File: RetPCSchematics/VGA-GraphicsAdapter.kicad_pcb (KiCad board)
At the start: 2 copper layers, 200.7 x 104.1 mm, 27 parts, among them U501 TFP410, U8 SN74LVC245AN, X1 DGOF5S3

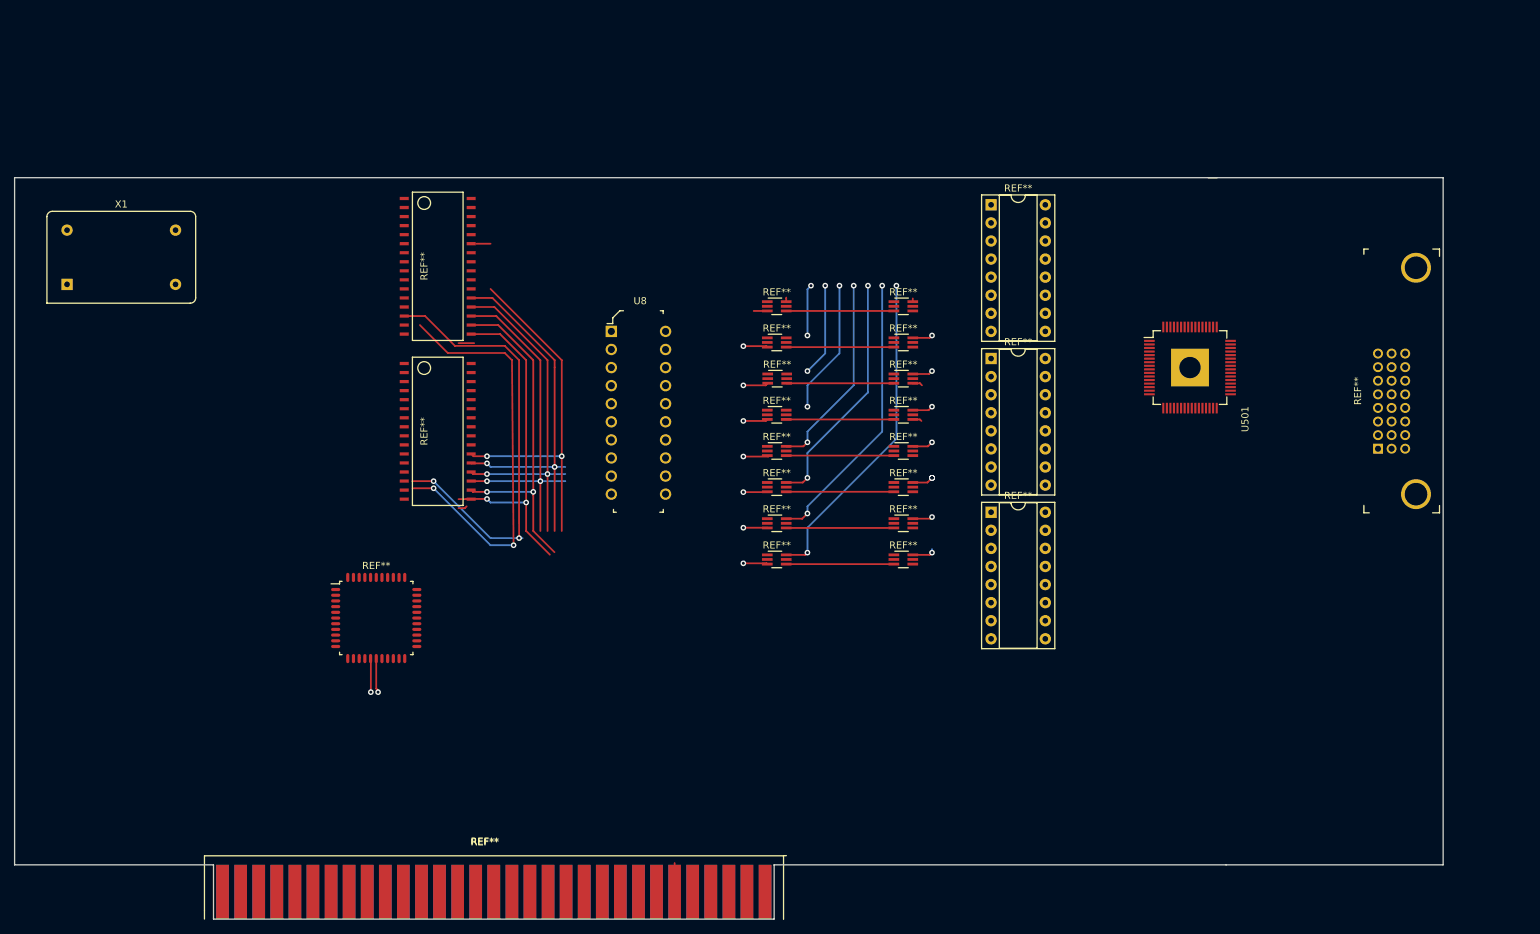
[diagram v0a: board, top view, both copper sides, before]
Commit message: sync
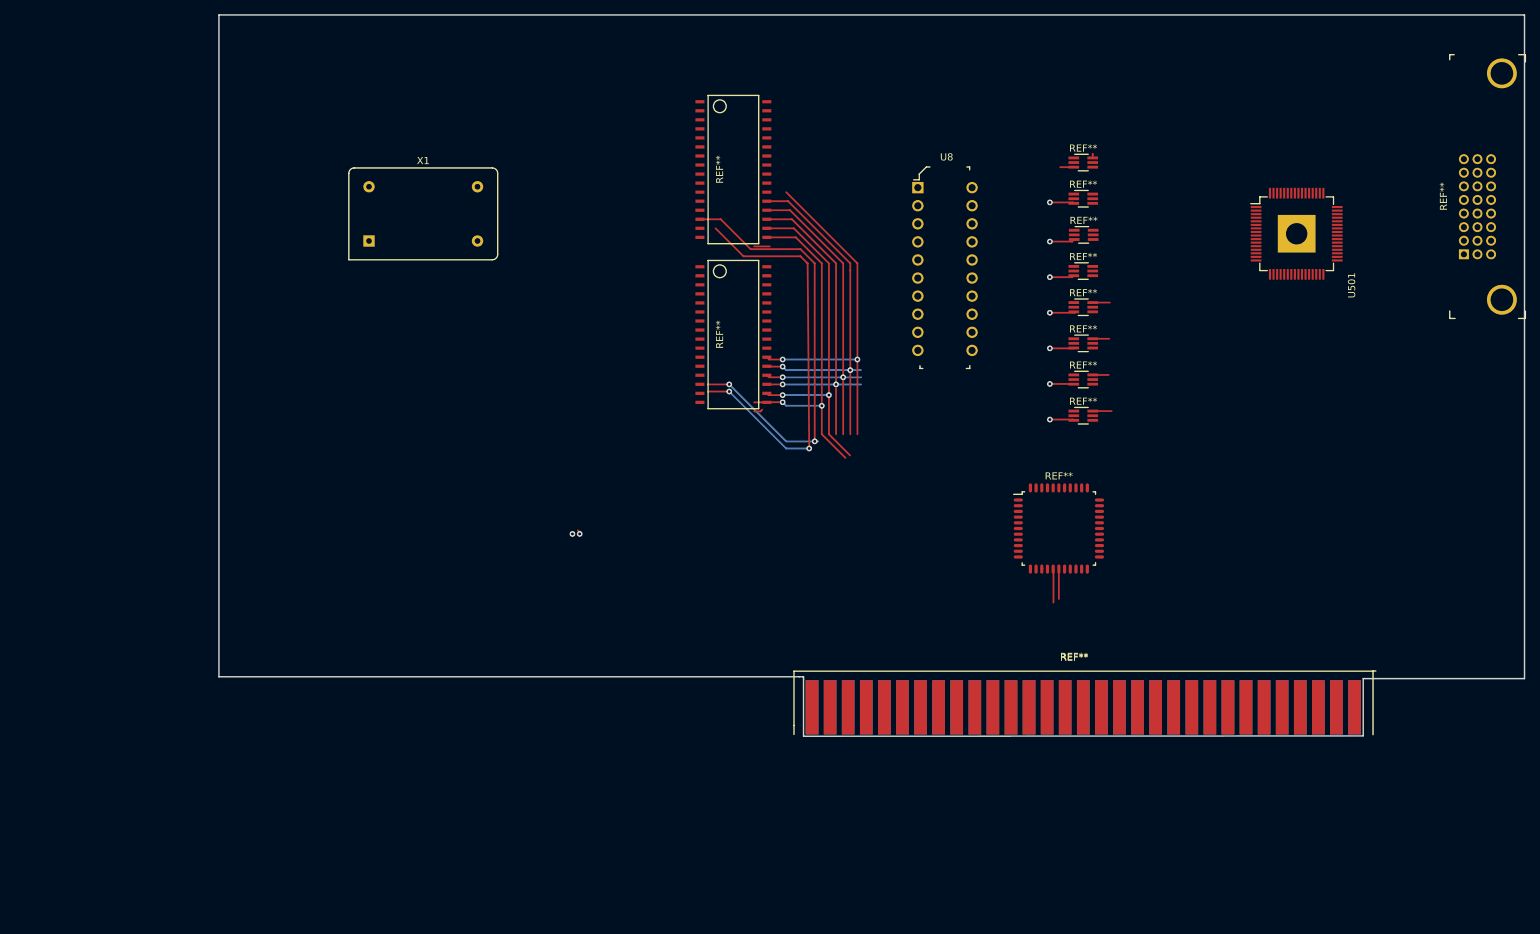
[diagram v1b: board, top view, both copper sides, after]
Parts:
- removed the REF** at (172.7, 115.6)
- removed the REF** at (160.4, 107.0)
- removed the REF** at (160.4, 101.9)
- removed the REF** at (160.4, 96.8)
- removed the REF** at (160.4, 91.7)
- removed the REF** at (160.4, 86.6)
- removed the REF** at (142.6, 112.0)
- removed the REF** at (142.6, 107.0)
- removed the REF** at (142.6, 101.9)
- removed the REF** at (142.7, 96.8)
- removed the REF** at (142.6, 91.7)
- removed the REF** at (172.7, 72.4)
- removed the REF** at (172.7, 94.0)
- removed the REF** at (160.4, 122.2)
- removed the REF** at (160.4, 117.1)
- removed the REF** at (142.6, 122.2)
- removed the REF** at (142.6, 117.1)
- removed the REF** at (160.4, 112.0)
- added REF**: SOT-363_SC-70-6_Handsoldering, Package_TO_SOT_SMD:SOT-363_SC-70-6_Handsoldering, F.Cu at (185.7, 102.0)
- added REF**: SOT-363_SC-70-6_Handsoldering, Package_TO_SOT_SMD:SOT-363_SC-70-6_Handsoldering, F.Cu at (185.7, 96.9)
- added REF**: SOT-363_SC-70-6_Handsoldering, Package_TO_SOT_SMD:SOT-363_SC-70-6_Handsoldering, F.Cu at (185.7, 91.9)
- added REF**: SOT-363_SC-70-6_Handsoldering, Package_TO_SOT_SMD:SOT-363_SC-70-6_Handsoldering, F.Cu at (185.7, 86.8)
- added REF**: SOT-363_SC-70-6_Handsoldering, Package_TO_SOT_SMD:SOT-363_SC-70-6_Handsoldering, F.Cu at (185.7, 81.7)
- added REF**: SOT-363_SC-70-6_Handsoldering, Package_TO_SOT_SMD:SOT-363_SC-70-6_Handsoldering, F.Cu at (185.7, 76.6)
- added REF**: SOT-363_SC-70-6_Handsoldering, Package_TO_SOT_SMD:SOT-363_SC-70-6_Handsoldering, F.Cu at (185.7, 71.5)
- moved REF** 96.7 mm to (182.2, 117.9)
- moved REF** 86.8 mm to (184.4, 135.4)
- moved REF** 47.6 mm to (185.7, 66.5)
- moved U8 47.6 mm to (162.4, 70.0)
- moved REF** 43.7 mm to (136.5, 67.4)
- moved REF** 43.7 mm to (136.5, 90.6)
- moved X1 42.9 mm to (85.3, 77.5)
- moved REF** 29.9 mm to (244.5, 85.7)
- moved U501 24.0 mm to (215.6, 76.5)
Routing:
- net (no net): track 796.9 -> 473.6 mm, vias 48 -> 25
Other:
- board size 200.7 x 104.1 mm -> 183.4 x 101.3 mm
